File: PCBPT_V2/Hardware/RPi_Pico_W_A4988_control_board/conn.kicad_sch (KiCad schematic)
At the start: 40 parts, among them J1 Limit Switch, J10 Limit Switch, J11 Limit Switch, J12 Limit Switch, J19 Limit Switch, J2 Limit Switch, J20 Conn_01x06_Pin, J21 Conn_01x06_Pin, J22 Limit Switch, J3 Limit Switch, J4 Limit Switch, J5 Limit Switch, J6 Limit Switch, J7 Limit Switch, J8 Limit Switch, J9 Limit Switch

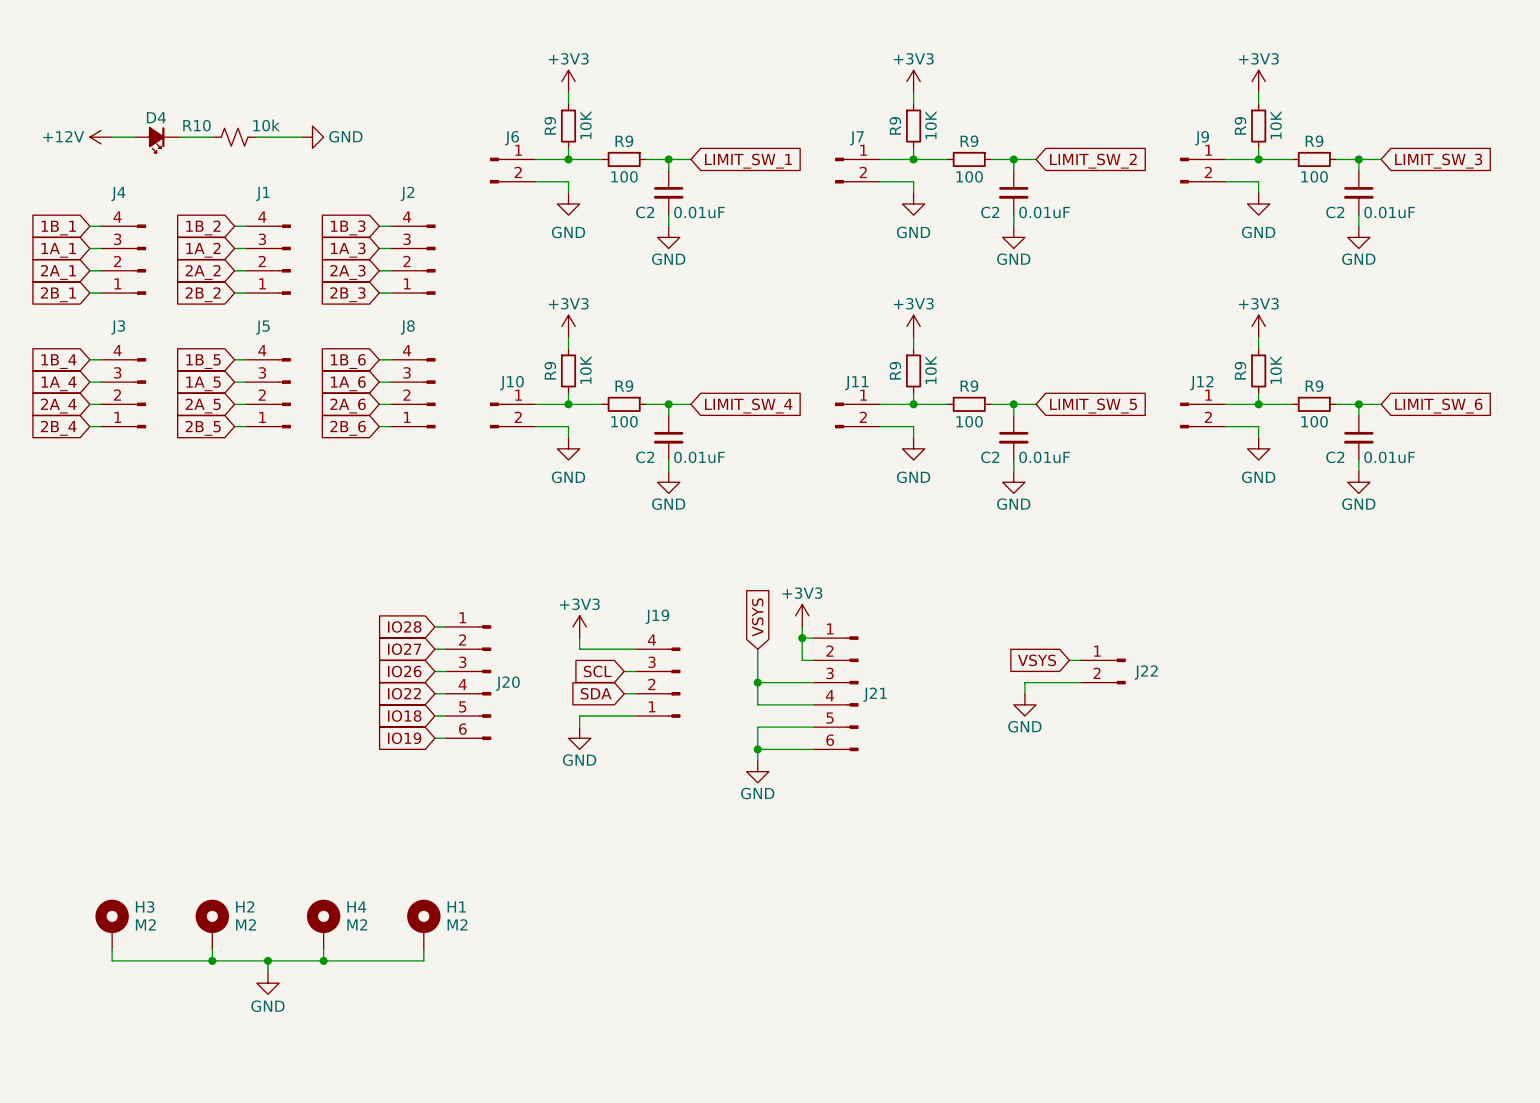
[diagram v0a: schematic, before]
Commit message: udated by FZ
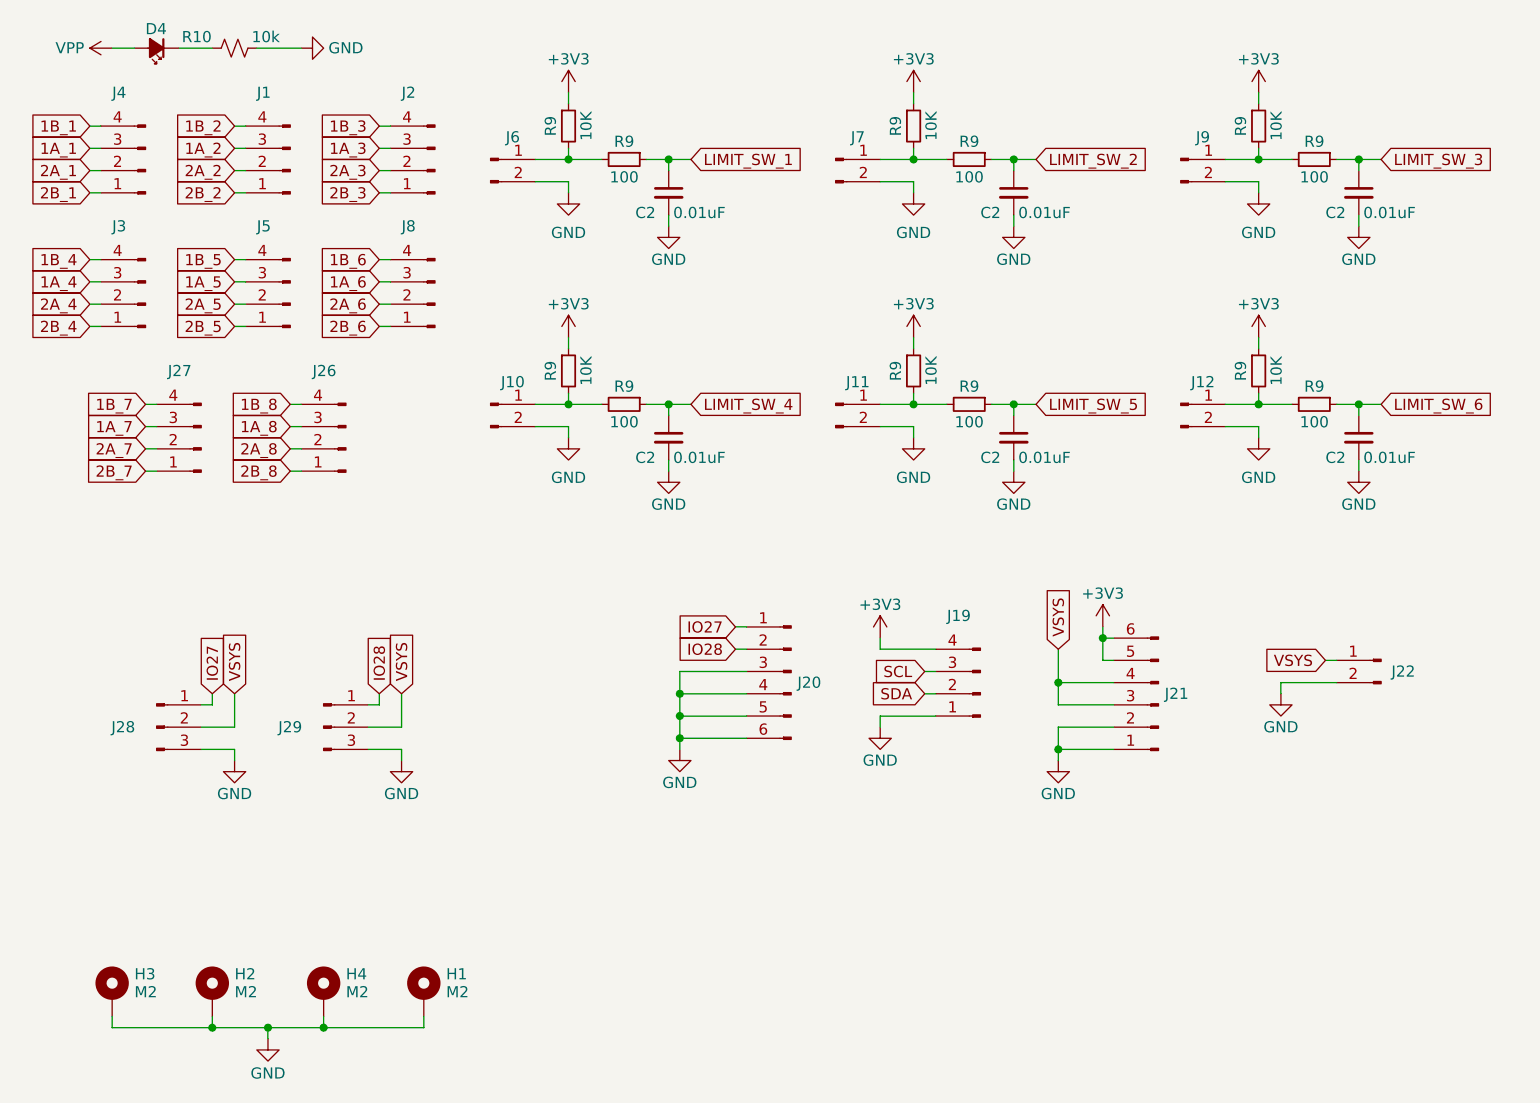
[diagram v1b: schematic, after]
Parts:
- added J26, J27: Limit Switch, Connector_PinHeader_2.54mm:PinHeader_1x04_P2.54mm_Vertical, symbol Connector:Conn_01x04_Male
- added J28, J29: Conn_01x03_Pin, Connector_PinHeader_2.54mm:PinHeader_1x03_P2.54mm_Vertical, symbol Connector:Conn_01x03_Pin
- C2: footprint Capacitor_SMD:C_0603_1608Metric_Pad1.08x0.95mm_HandSolder -> Capacitor_SMD:C_1206_3216Metric_Pad1.33x1.80mm_HandSolder
- D4: footprint LED_SMD:LED_0603_1608Metric -> LED_SMD:LED_1206_3216Metric_Pad1.42x1.75mm_HandSolder
- J20, J21: footprint (none) -> Connector_PinHeader_2.54mm:PinHeader_1x06_P2.54mm_Vertical
- R10: footprint Resistor_SMD:R_0603_1608Metric -> Resistor_SMD:R_1206_3216Metric_Pad1.30x1.75mm_HandSolder
- R9: footprint Resistor_SMD:R_0603_1608Metric_Pad0.98x0.95mm_HandSolder -> Resistor_SMD:R_1206_3216Metric_Pad1.30x1.75mm_HandSolder
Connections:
- net IO18 is gone; now on net GND: J20.5 (Pin_5)
- net IO19 is gone; now on net GND: J20.6 (Pin_6)
- net IO22 is gone; now on net GND: J20.4 (Pin_4)
- net IO26 is gone; now on net GND: J20.3 (Pin_3)
- net +3V3: now also J21.5 (Pin_5), J21.6 (Pin_6); no longer J21.1 (Pin_1), J21.2 (Pin_2)
- net GND: now also J21.1 (Pin_1), J21.2 (Pin_2), J28.3 (Pin_3), J29.3 (Pin_3); no longer J21.5 (Pin_5), J21.6 (Pin_6)
- net IO27: now also J20.1 (Pin_1), J28.1 (Pin_1); no longer J20.2 (Pin_2)
- net IO28: now also J20.2 (Pin_2), J29.1 (Pin_1); no longer J20.1 (Pin_1)
- net VSYS: now also J28.2 (Pin_2), J29.2 (Pin_2)
- net +12V renamed VPP
- new net 1A_7: J27.3 (Pin_3)
- new net 1A_8: J26.3 (Pin_3)
- new net 1B_7: J27.4 (Pin_4)
- new net 1B_8: J26.4 (Pin_4)
- new net 2A_7: J27.2 (Pin_2)
- new net 2A_8: J26.2 (Pin_2)
- new net 2B_7: J27.1 (Pin_1)
- new net 2B_8: J26.1 (Pin_1)
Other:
- moved on the sheet: D4, H1, H2, H3, H4, J1, J19, J2, J20, J21, J22, J3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
